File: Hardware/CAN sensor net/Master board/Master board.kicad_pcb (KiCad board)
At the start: 2 copper layers, 47.2 x 28.9 mm, 74 parts, among them J1 Micro_SD_Card_Con, J2 USB_B_Micro, J3 Conn_02x05_SWD, J4 XT60, J5 532610671, J6 532610671, SW1 SW_Push, SW2 SW_SPDT, U1 STM32F405RGTx, U2 USBLC6-2SC6, U3 ST1S14PHR, U4 LDL1117_3V3, U5 SN65HVD230, U6 SN65HVD230, U7 W25Q32FVSSIG, Y1 16MHz

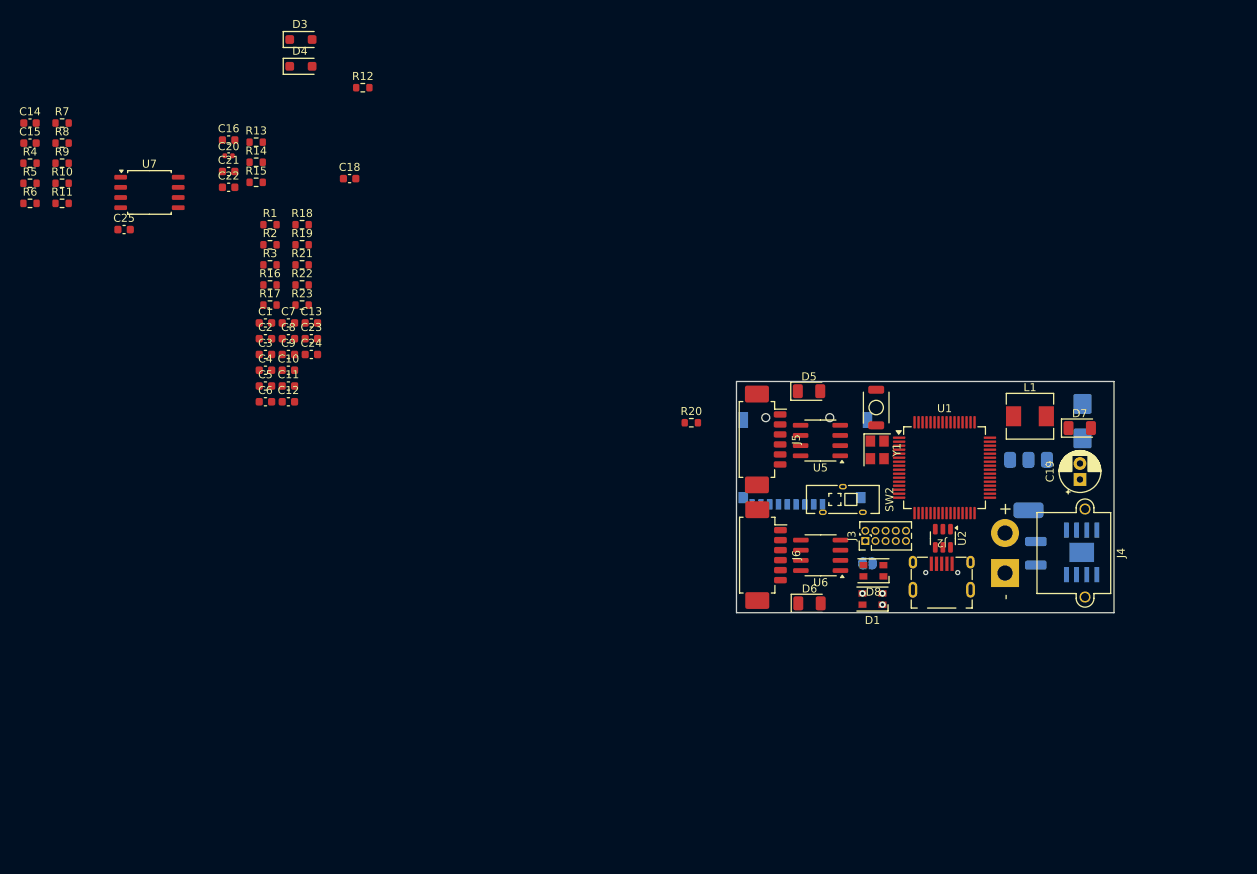
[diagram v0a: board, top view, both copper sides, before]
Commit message: Bugfix
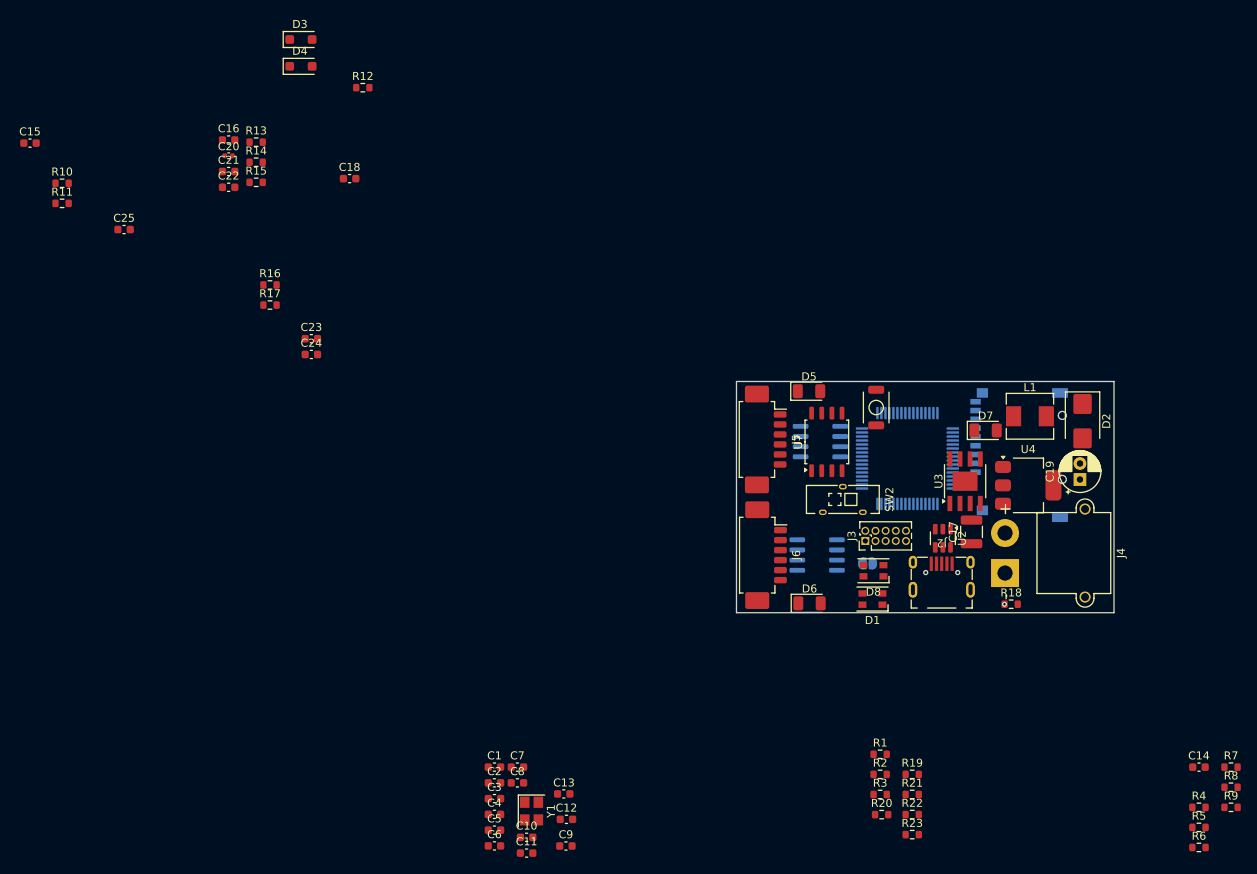
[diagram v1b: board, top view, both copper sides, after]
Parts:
- C17, D2, U3, U4: moved to F.Cu
- U1, U5, U6: moved to B.Cu
- moved C14 166.8 mm to (228.0, 132.3)
- moved R4 166.8 mm to (228.0, 137.4)
- moved R5 166.8 mm to (228.0, 139.9)
- moved R6 166.8 mm to (228.0, 142.4)
- moved R7 166.8 mm to (232.0, 132.3)
- moved R8 166.8 mm to (232.0, 134.8)
- moved R9 166.8 mm to (232.0, 137.4)
- moved R1 101.0 mm to (188.1, 130.7)
- moved R19 101.0 mm to (192.1, 133.2)
- moved R2 101.0 mm to (188.1, 133.2)
- moved R21 101.0 mm to (192.1, 135.7)
- moved R22 101.0 mm to (192.1, 138.3)
- moved R23 101.0 mm to (192.1, 140.8)
- moved R3 101.0 mm to (188.1, 135.7)
- moved R18 100.5 mm to (204.5, 112.0)
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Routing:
- net Net-(D5-K): vias 0 -> 1
- net Net-(D1-RK): vias 1 -> 0
- net Net-(D1-GK): vias 1 -> 0
- net Net-(D1-BK): vias 1 -> 0
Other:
- board text added: "led"
- board text added: "разъём программатора юарт??"
